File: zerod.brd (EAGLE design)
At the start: 82.2 x 80 mm, 38 parts, among them IC1 NE5532N, IC2 LM3914N, Q1 2N3906

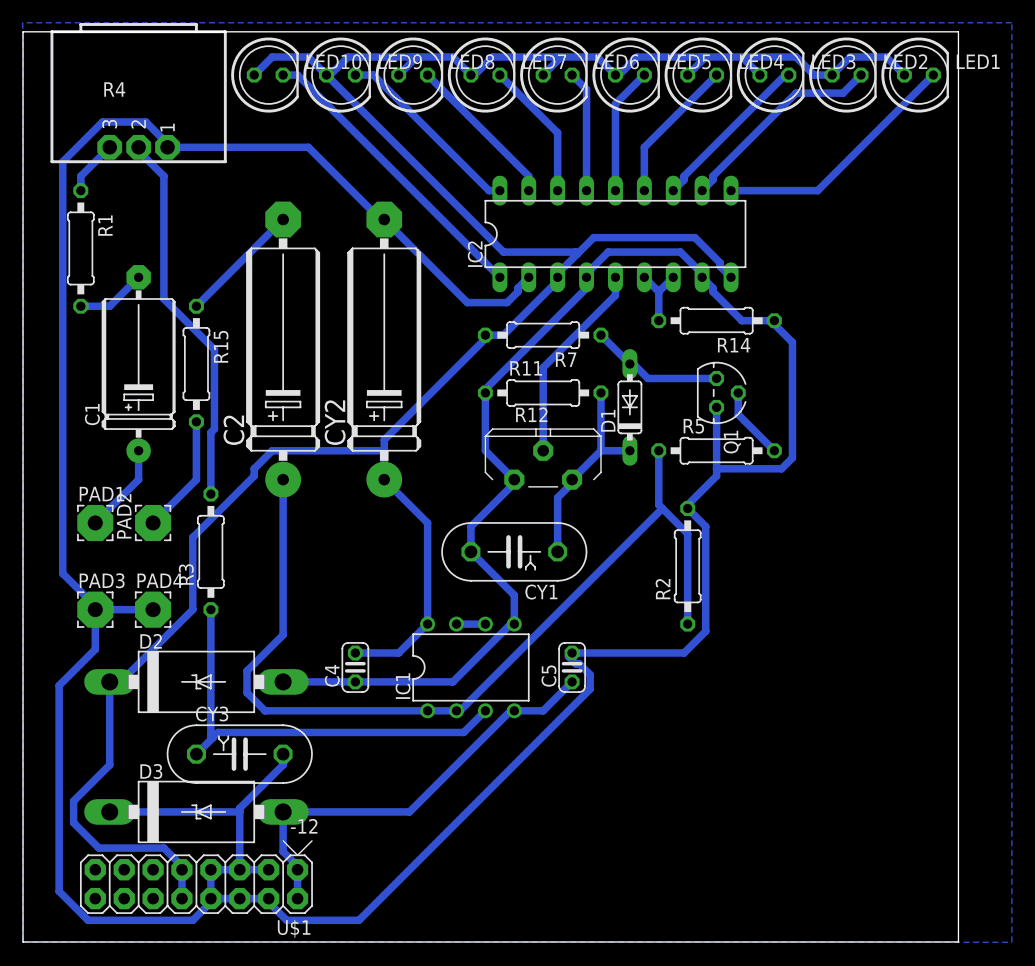
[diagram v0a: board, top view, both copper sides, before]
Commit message: new, smaller board
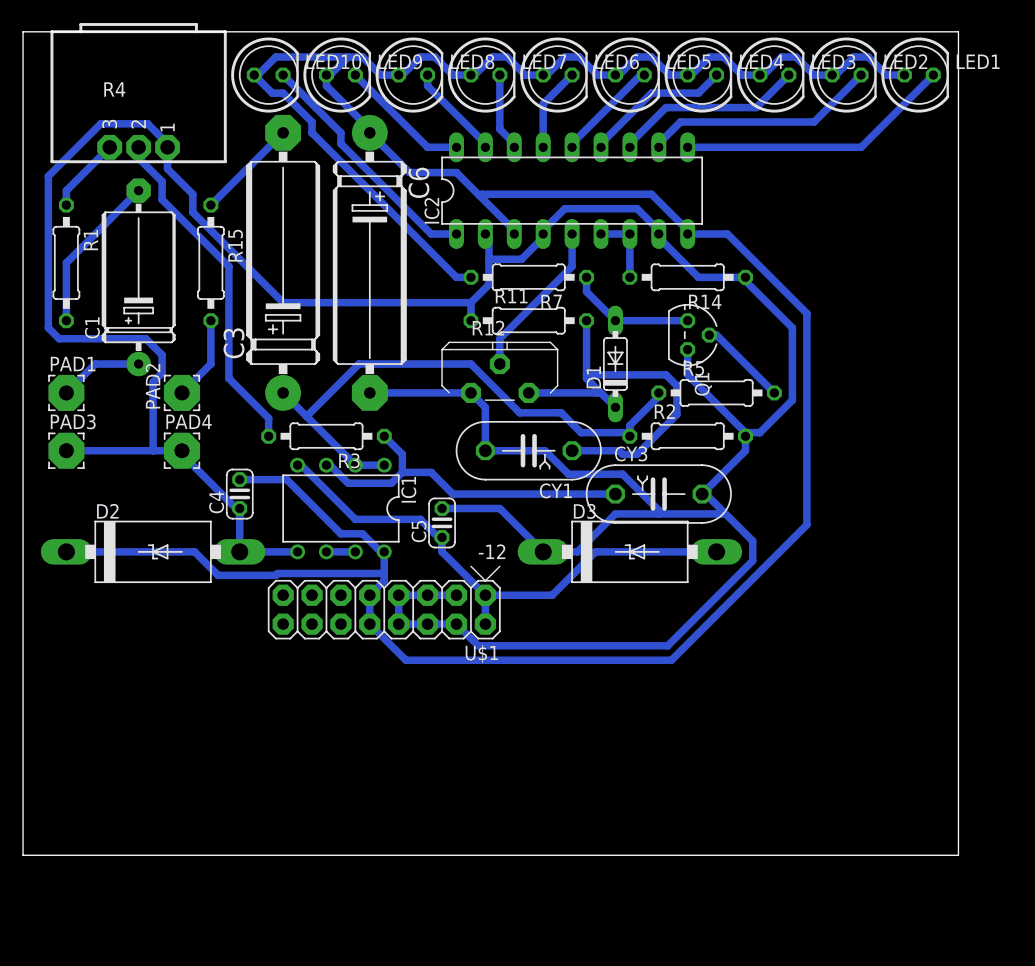
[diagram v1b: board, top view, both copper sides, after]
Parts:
- removed C2: 100uF, rcl:E22-6
- removed CY2: 10uF, rcl:E22-6
- added C3: 100uF, rcl:E22-6
- added C6: 10uF, rcl:E22-6
- moved D3 44.4 mm to (53.3, 34.3)
- moved CY3 43.3 mm to (55.9, 39.4)
- moved U$1 29.2 mm to (34.3, 29.2)
- moved C4 18.3 mm to (19.1, 39.4)
- moved IC1 18.1 mm to (27.9, 38.1), turned to 180 degrees
- moved C5 17.1 mm to (36.8, 36.8)
- moved R3 14.4 mm to (26.7, 44.5), turned to 180 degrees
- moved PAD4 14.2 mm to (14.0, 43.2)
- moved PAD3 14.2 mm to (3.81, 43.2)
- moved D2 12.0 mm to (11.4, 34.3)
- moved PAD1 11.7 mm to (3.81, 48.3)
- moved PAD2 11.7 mm to (14.0, 48.3)
- moved R2 11.4 mm to (58.4, 44.5), turned to 0 degrees
- moved CY1 8.98 mm to (44.5, 43.2)
- moved R15 8.98 mm to (16.5, 59.7)
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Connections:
- net +12V: now also C6.+; no longer CY2.+
- net GNDA: now also C6.-; no longer CY2.-
- net N$3: now also C3.-; no longer C2.-
- net N$5: now also C3.+; no longer C2.+
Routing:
- net GNDA: track 350.1 -> 288.2 mm
- net +12V: track 230.5 -> 268.1 mm
- net N$5: track 80.9 -> 49.3 mm
- net N$12: track 18.1 -> 36.6 mm
- net -12V: track 38.3 -> 46.4 mm
- net N$2: track 6.13 -> 14.1 mm
- net N$6: track 38.3 -> 31.1 mm
- net N$21: track 13.8 -> 8.45 mm
- net N$20: track 12.3 -> 6.88 mm
- net N$22: track 16.9 -> 11.5 mm
- net N$23: track 26.4 -> 21.6 mm
- net N$10: track 17.9 -> 14.1 mm
- net N$19: track 10.7 -> 7.40 mm
- net N$7: track 33.4 -> 30.1 mm
- net N$8: track 10.5 -> 7.40 mm
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- removed copper zone on layer 16, net _OUTLINES_
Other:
- board size 82.2 x 80 mm -> 82.2 x 72.4 mm
